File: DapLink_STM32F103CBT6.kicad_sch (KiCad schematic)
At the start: 0 parts

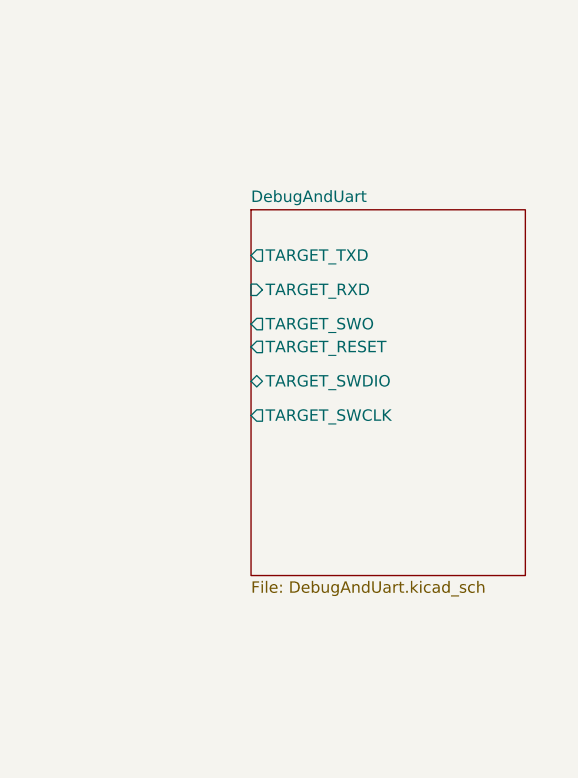
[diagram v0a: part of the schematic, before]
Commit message: temp
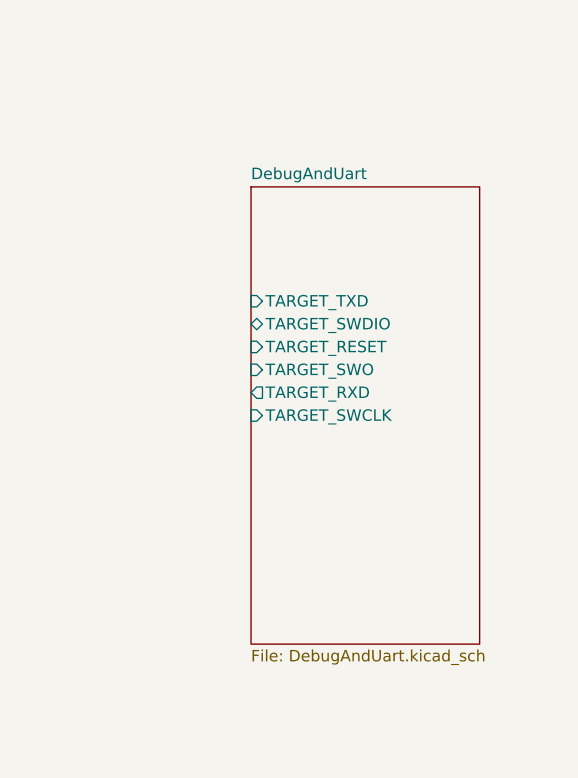
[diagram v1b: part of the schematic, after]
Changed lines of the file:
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@@
 	)
 	(sheet
-		(at 228.6 78.74)
-		(size 30.48 40.64)
+		(at 228.6 76.2)
+		(size 25.4 50.8)
 		(fields_autoplaced yes)
 		(stroke
@@
 		)
 		(property "Sheetname" "DebugAndUart"
-			(at 228.6 78.0284 0)
+			(at 228.6 75.4884 0)
 			(effects
 				(font
@@
 		)
 		(property "Sheetfile" "DebugAndUart.kicad_sch"
-			(at 228.6 119.9646 0)
+			(at 228.6 127.5846 0)
 			(effects
 				(font
@@
 			)
 		)
-		(pin "TARGET_TXD" output
-			(at 228.6 83.82 180)
+		(pin "TARGET_TXD" input
+			(at 228.6 88.9 180)
 			(effects
 				(font
@@
 			)
 		)
-		(pin "TARGET_RXD" input
-			(at 228.6 87.63 180)
-			(effects
-				(font
-					(size 1.27 1.27)
-				)
-				(justify left)
-			)
-		)
-		(pin "TARGET_SWO" output
+		(pin "TARGET_SWDIO" bidirectional
 			(at 228.6 91.44 180)
 			(effects
@@
 			)
 		)
-		(pin "TARGET_RESET" output
+		(pin "TARGET_RESET" input
 			(at 228.6 93.98 180)
 			(effects
@@
 			)
 		)
-		(pin "TARGET_SWDIO" bidirectional
-			(at 228.6 97.79 180)
+		(pin "TARGET_SWO" input
+			(at 228.6 96.52 180)
 			(effects
 				(font
@@
 			)
 		)
-		(pin "TARGET_SWCLK" output
+		(pin "TARGET_RXD" output
+			(at 228.6 99.06 180)
+			(effects
+				(font
+					(size 1.27 1.27)
+				)
+				(justify left)
+			)
+		)
+		(pin "TARGET_SWCLK" input
 			(at 228.6 101.6 180)
 			(effects
